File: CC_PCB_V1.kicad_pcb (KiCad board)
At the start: 2 copper layers, 11 parts, among them J2 Antenna_Conn_02x04_Odd_Even, J3 USB1130-15-A_REVA, J5 Relay_Conn_01x06, U1 Pico, U2 level_converter_BOB-12009

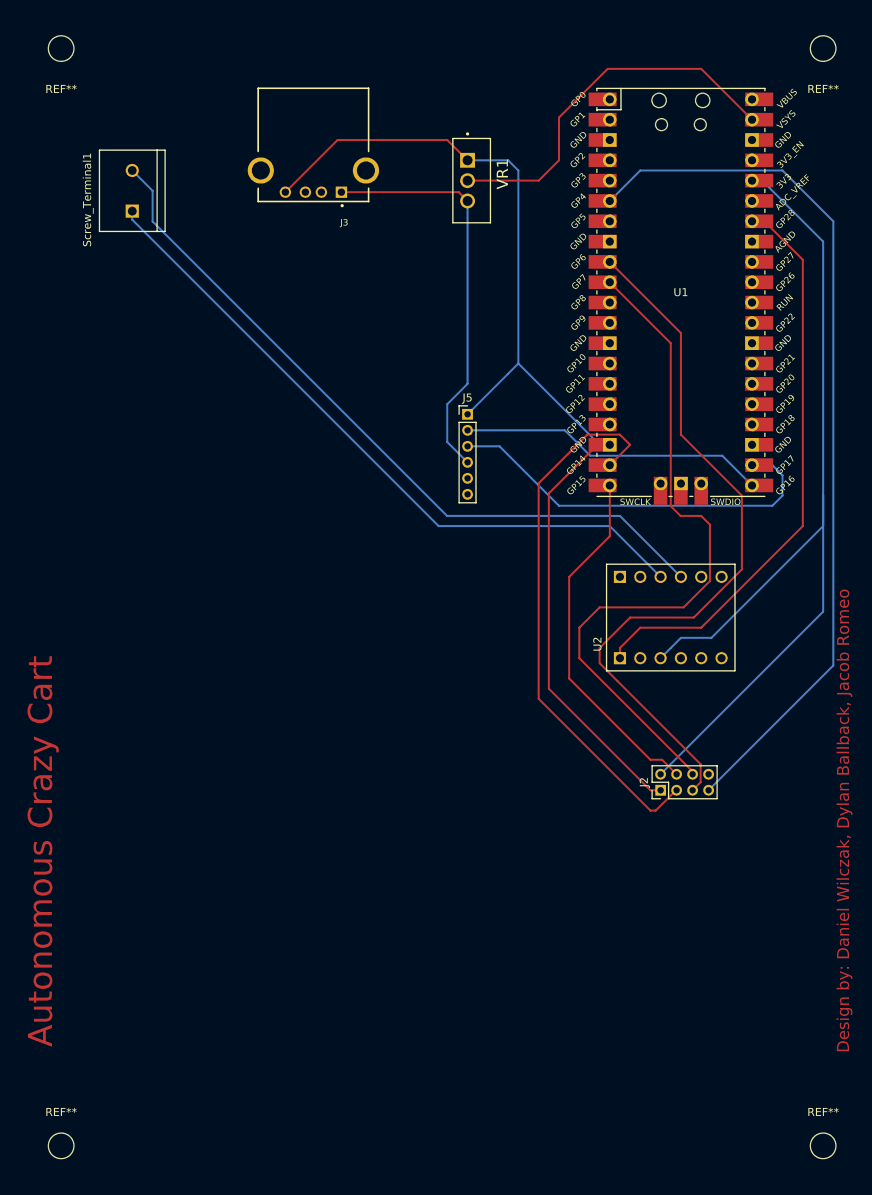
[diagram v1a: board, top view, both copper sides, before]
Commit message: Completed V1 PCB
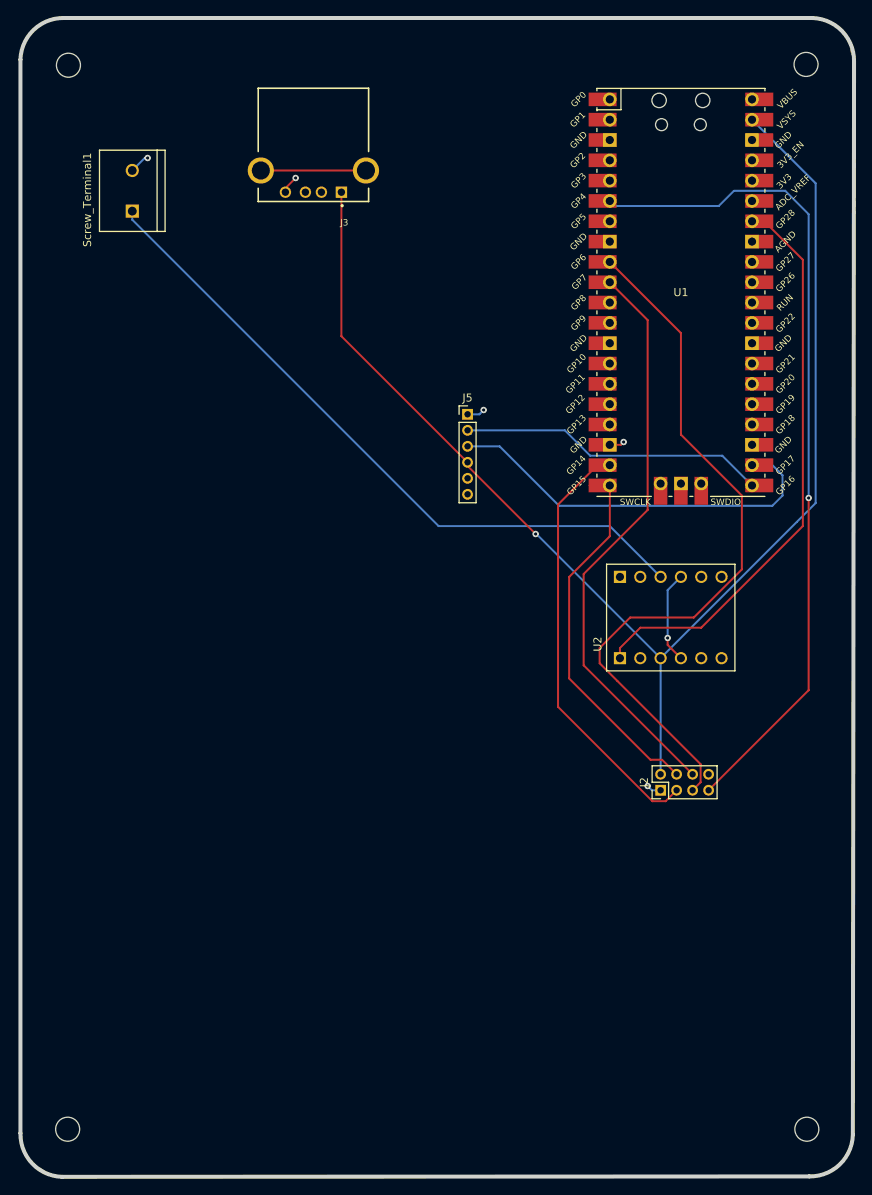
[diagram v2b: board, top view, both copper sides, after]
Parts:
- removed the REF** at (154.9, 20.3)
- removed the REF** at (59.7, 20.3)
- removed the REF** at (154.9, 157.5)
- removed the REF** at (59.7, 157.5)
- removed VR1: LM1117T-3.3_NOPB, MCU_RaspberryPi_and_Boards:TO254P1054X470X1955-3
- added REF**: MountingHole_3mm, MountingHole:MountingHole_3mm, F.Cu at (152.9, 155.4)
- added REF**: MountingHole_3mm, MountingHole:MountingHole_3mm, F.Cu at (60.5, 155.4)
- added REF**: MountingHole_3mm, MountingHole:MountingHole_3mm, F.Cu at (152.8, 22.3)
- added REF**: MountingHole_3mm, MountingHole:MountingHole_3mm, F.Cu at (60.6, 22.4)
- U2: footprint BOB-12009:CONV_BOB-12009 -> MCU_RaspberryPi_and_Boards:CONV_BOB-12009
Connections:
- J2 pad 2: +3V3 -> +5V
- Screw_Terminal1 pad 2: Net-(Screw_Terminal1-Pad2) -> GND
- U1 pad 36: +3V3 -> Net-(U1-Pad36)
- U1 pad 39: +3V3 -> +5V
- U2 pad GND_1: Net-(Screw_Terminal1-Pad2) -> GND
- U2 pad GND_2: Net-(Screw_Terminal1-Pad2) -> GND
- U2 pad LV: +3V3 -> +5V
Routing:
- net +3V3: track 166.7 -> 0.00 mm
- net +5V: track 51.0 -> 168.0 mm, vias 0 -> 1
- net GND: track 135.9 -> 22.3 mm, vias 0 -> 6
- net Net-(Screw_Terminal1-Pad2): track 91.9 -> 0.00 mm
- net GP14: track 69.1 -> 54.1 mm
- net GP7: track 87.0 -> 72.4 mm
- net Net-(J3-PadS1): track 0.00 -> 13.1 mm
- net GP4: track 109.7 -> 104.3 mm, vias 0 -> 1
- net Net-(U1-Pad36): track 0.00 -> 1.55 mm
- added copper zone on B.Cu, net GND
- added copper zone on F.Cu, net GND
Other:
- board outline added: 104.2 x 144.9 mm
- board text added: "Autonomous Crazy Cart V1"
- board text removed: "Autonomous Crazy Cart"
